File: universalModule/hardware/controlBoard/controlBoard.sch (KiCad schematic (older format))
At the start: 13 parts, among them J10 BATT_1, J11 BATT_3, J12 BATT_2, J13 PWR_1, J14 BATT_2, J15 PWR_3, J16 CTL_3, J17 CTL_1, J18 CTL_2, J19 PWR_4, J20 CTL_5, J21 CTL_4, J22 INT_1

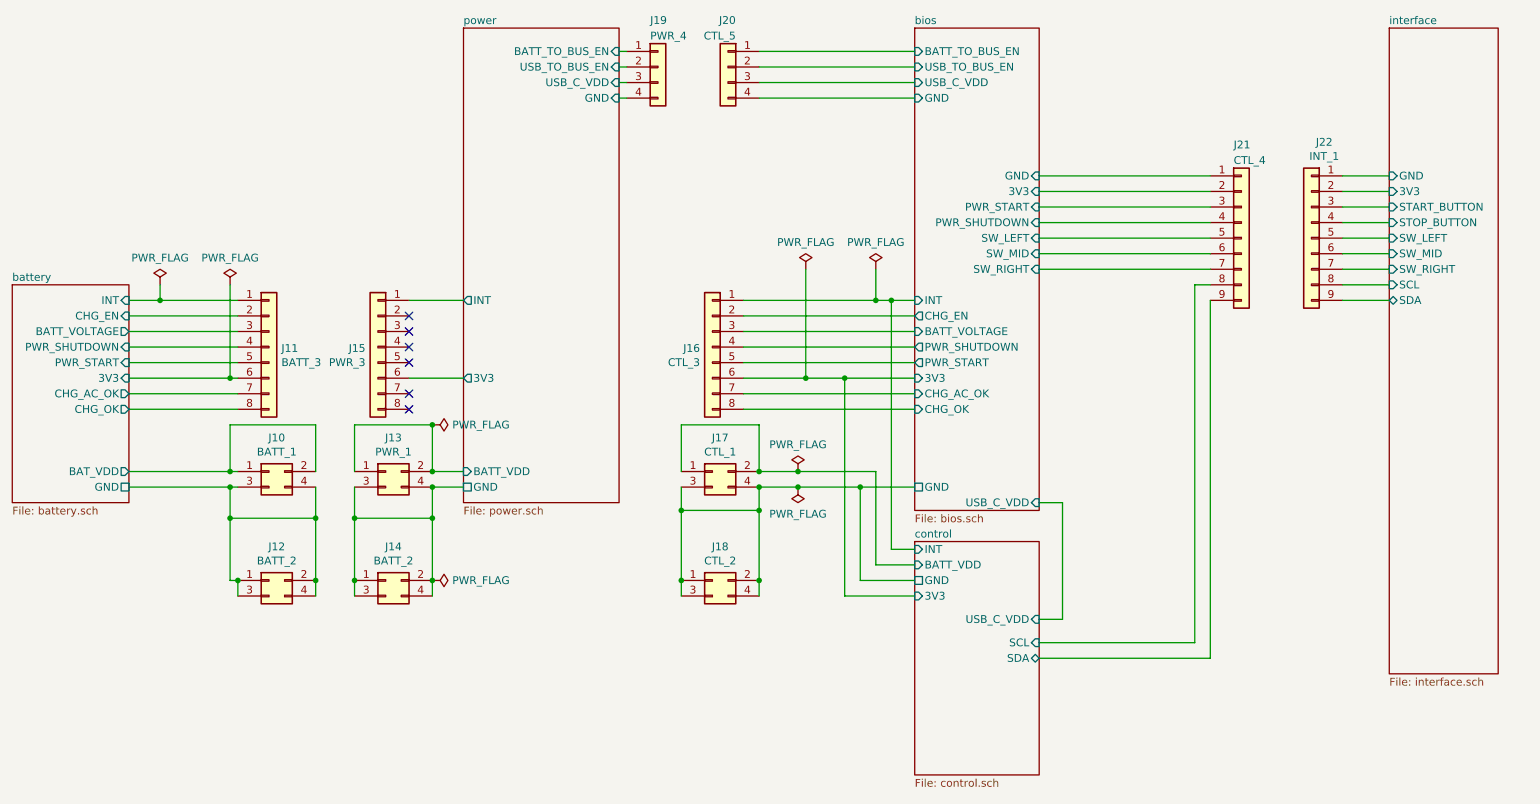
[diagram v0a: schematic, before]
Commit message: universalModule: Fine tune the control board
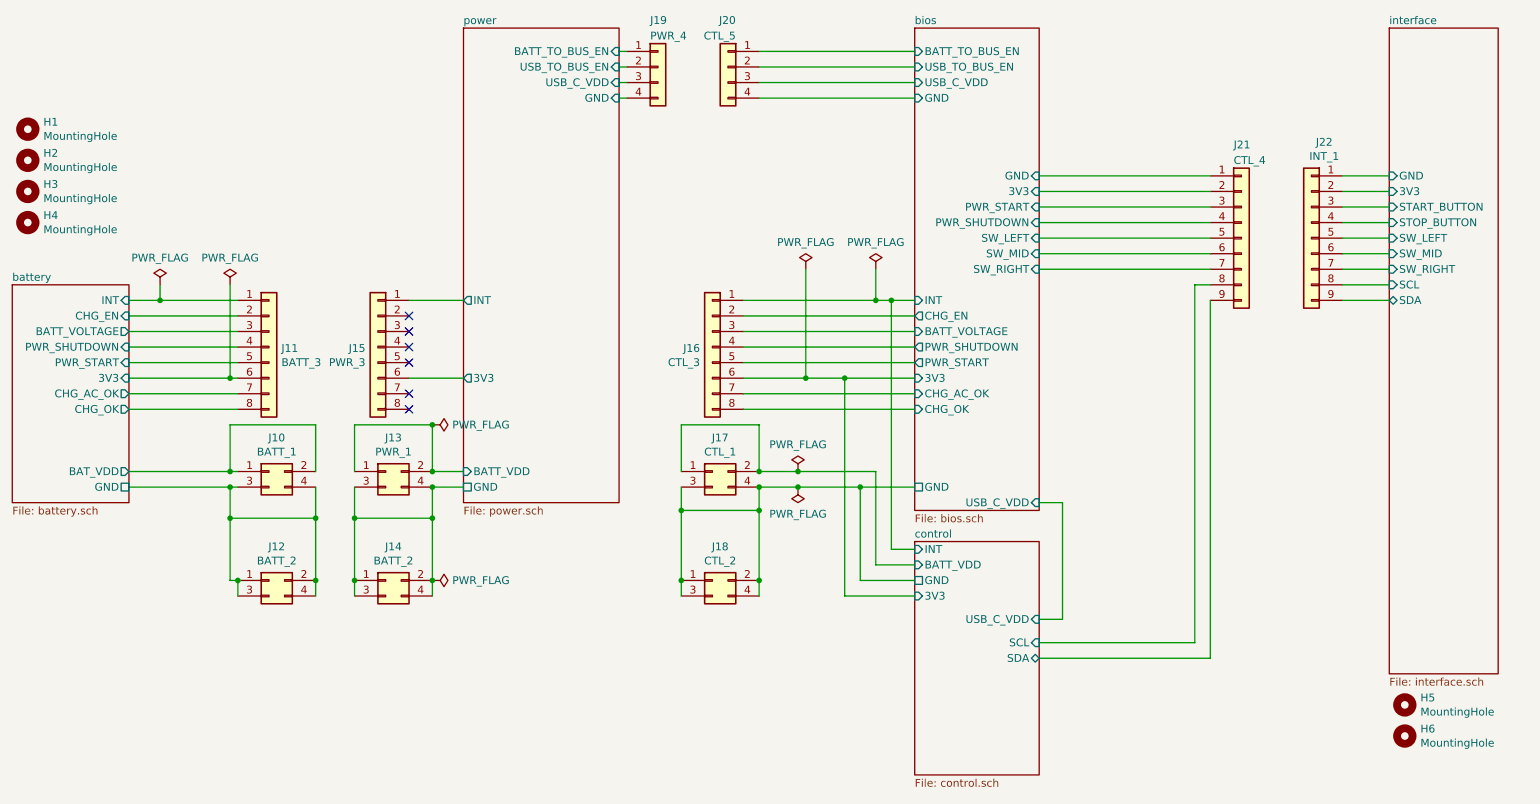
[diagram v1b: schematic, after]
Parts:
- added H1, H2, H3, H4, H5, H6: MountingHole, MountingHole:MountingHole_2.1mm, symbol Mechanical:MountingHole
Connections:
- net bios/3V3 is gone; now on net bios/3V3: J21.2 (Pin_2)
- net bios/GND is gone; now on net bios/GND: J20.4 (Pin_4)
- net bios/PWR_SHUTDOWN is gone; now on net bios/PWR_SHUTDOWN: J21.4 (Pin_4)
- net bios/PWR_START is gone; now on net bios/PWR_START: J21.3 (Pin_3)
- net bios/USB_C_VDD is gone; now on net bios/USB_C_VDD: J20.3 (Pin_3)
- net power/GND is gone; now on net power/GND: J19.4 (Pin_4)
- net bios/3V3: no longer J16.6 (Pin_6)
- net bios/GND: no longer J17.3 (Pin_3), J17.4 (Pin_4), J18.1 (Pin_1), J18.2 (Pin_2), J18.3 (Pin_3), J18.4 (Pin_4)
- net bios/PWR_SHUTDOWN: no longer J16.4 (Pin_4)
- net bios/PWR_START: no longer J16.5 (Pin_5)
- net power/GND: no longer J13.3 (Pin_3), J13.4 (Pin_4), J14.1 (Pin_1), J14.2 (Pin_2), J14.3 (Pin_3), J14.4 (Pin_4)
- new net bios/3V3: J16.6 (Pin_6)
- new net bios/GND: J17.3 (Pin_3), J17.4 (Pin_4), J18.1 (Pin_1), J18.2 (Pin_2), J18.3 (Pin_3), J18.4 (Pin_4)
- new net bios/PWR_SHUTDOWN: J16.4 (Pin_4)
- new net bios/PWR_START: J16.5 (Pin_5)
- new net power/GND: J13.3 (Pin_3), J13.4 (Pin_4), J14.1 (Pin_1), J14.2 (Pin_2), J14.3 (Pin_3), J14.4 (Pin_4)
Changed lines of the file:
@@
 Wire Wire Line
 	6000 3200 6450 3200
+$Comp
+L Mechanical:MountingHole H4
+U 1 1 5DE07B9A
+P 750 2200
+F 0 "H4" H 850 2246 50  0000 L CNN
+F 1 "MountingHole" H 850 2155 50  0000 L CNN
+F 2 "MountingHole:MountingHole_2.1mm" H 750 2200 50  0001 C CNN
+F 3 "~" H 750 2200 50  0001 C CNN
+	1    750  2200
+	1    0    0    -1
+$EndComp
+$Comp
+L Mechanical:MountingHole H3
+U 1 1 5DE0904B
+P 750 2000
+F 0 "H3" H 850 2046 50  0000 L CNN
+F 1 "MountingHole" H 850 1955 50  0000 L CNN
+F 2 "MountingHole:MountingHole_2.1mm" H 750 2000 50  0001 C CNN
+F 3 "~" H 750 2000 50  0001 C CNN
+	1    750  2000
+	1    0    0    -1
+$EndComp
+$Comp
+L Mechanical:MountingHole H2
+U 1 1 5DE091EE
+P 750 1800
+F 0 "H2" H 850 1846 50  0000 L CNN
+F 1 "MountingHole" H 850 1755 50  0000 L CNN
+F 2 "MountingHole:MountingHole_2.1mm" H 750 1800 50  0001 C CNN
+F 3 "~" H 750 1800 50  0001 C CNN
+	1    750  1800
+	1    0    0    -1
+$EndComp
+$Comp
+L Mechanical:MountingHole H1
+U 1 1 5DE0947E
+P 750 1600
+F 0 "H1" H 850 1646 50  0000 L CNN
+F 1 "MountingHole" H 850 1555 50  0000 L CNN
+F 2 "MountingHole:MountingHole_2.1mm" H 750 1600 50  0001 C CNN
+F 3 "~" H 750 1600 50  0001 C CNN
+	1    750  1600
+	1    0    0    -1
+$EndComp
+$Comp
+L Mechanical:MountingHole H5
+U 1 1 5DE0BB0E
+P 9600 5300
+F 0 "H5" H 9700 5346 50  0000 L CNN
+F 1 "MountingHole" H 9700 5255 50  0000 L CNN
+F 2 "MountingHole:MountingHole_2.1mm" H 9600 5300 50  0001 C CNN
+F 3 "~" H 9600 5300 50  0001 C CNN
+	1    9600 5300
+	1    0    0    -1
+$EndComp
+$Comp
+L Mechanical:MountingHole H6
+U 1 1 5DE0DC9E
+P 9600 5500
+F 0 "H6" H 9700 5546 50  0000 L CNN
+F 1 "MountingHole" H 9700 5455 50  0000 L CNN
+F 2 "MountingHole:MountingHole_2.1mm" H 9600 5500 50  0001 C CNN
+F 3 "~" H 9600 5500 50  0001 C CNN
+	1    9600 5500
+	1    0    0    -1
+$EndComp
 $EndSCHEMATC
